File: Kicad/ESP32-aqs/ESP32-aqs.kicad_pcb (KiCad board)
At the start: 2 copper layers, 22 parts, among them J1 UART Connector, J2 Conn SEN55, J3 ufl connector, U1 LD1117S33TR_SOT223, U2 ESP32-WROOM-32, U3 SGP41-D-R4, U4 SX1276S8S+T-X1

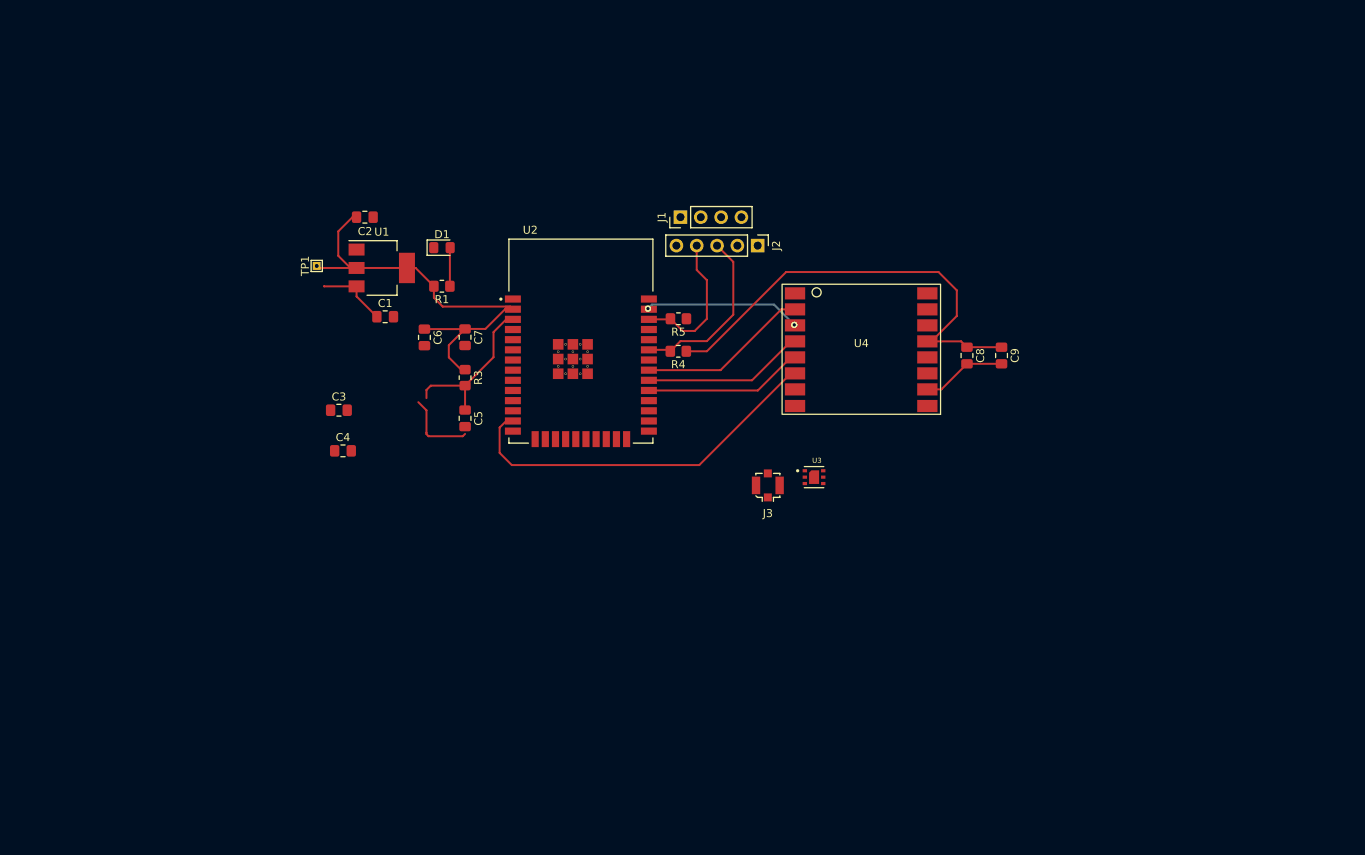
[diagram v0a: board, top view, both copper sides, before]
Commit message: PCB design update
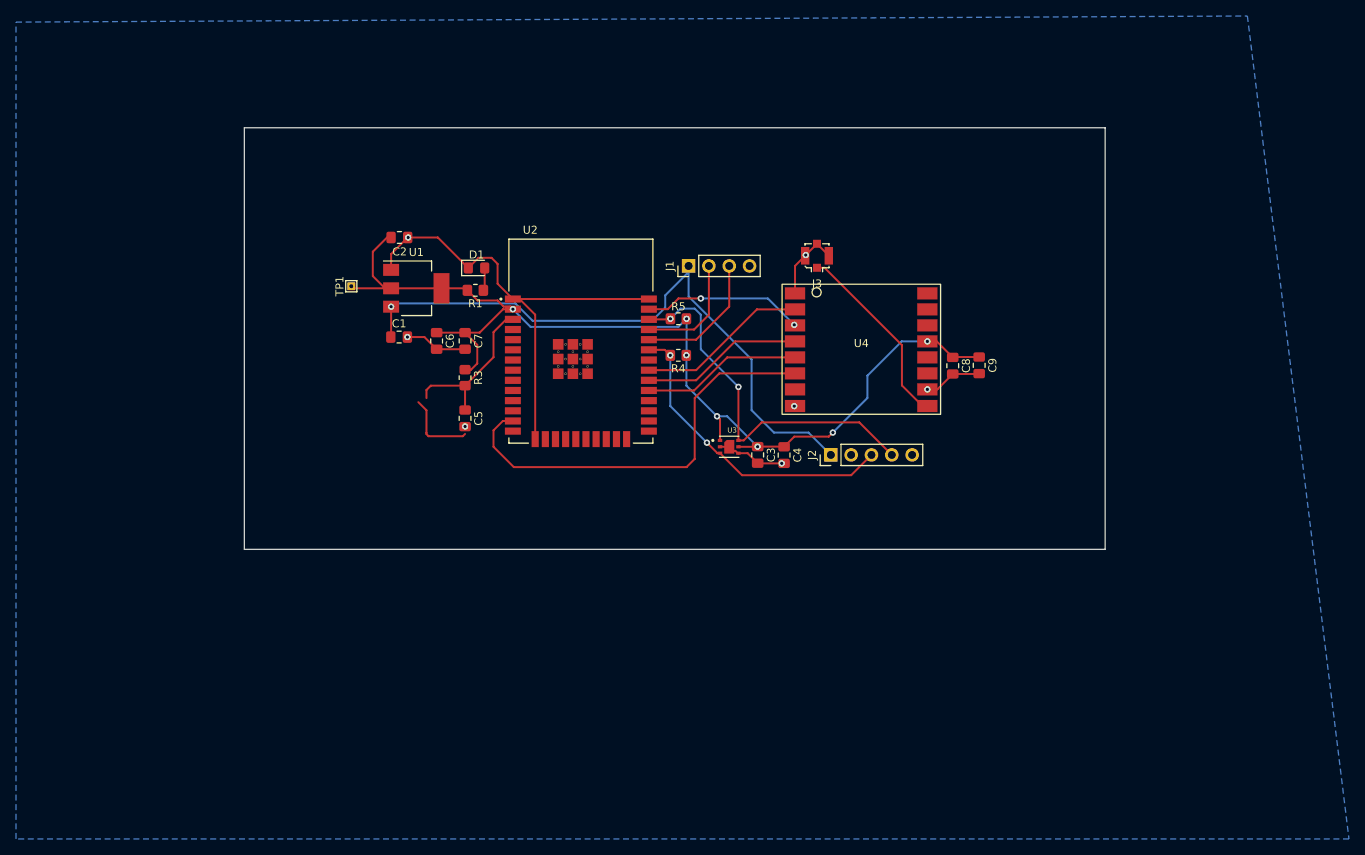
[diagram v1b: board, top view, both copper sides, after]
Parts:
- moved C4 55.1 mm to (182.4, 101.6), turned to -90 degrees
- moved C3 52.6 mm to (179.1, 101.6), turned to -90 degrees
- moved J3 29.4 mm to (186.5, 76.7)
- moved J2 27.7 mm to (188.2, 101.6), turned to 90 degrees
- moved U3 11.3 mm to (175.5, 100.6)
- moved J1 6.18 mm to (170.4, 78.0)
- moved D1 5.01 mm to (143.9, 78.2)
- moved TP1 5.01 mm to (128.3, 80.5)
- moved C2 5.01 mm to (134.3, 74.4)
- moved U1 5.01 mm to (136.4, 80.8)
- moved R1 4.21 mm to (143.8, 81.0)
- moved C1 3.08 mm to (134.2, 86.9)
- moved C9 3.05 mm to (206.8, 90.4)
- moved C8 2.18 mm to (203.5, 90.4)
- moved C6 1.59 mm to (138.9, 87.4)
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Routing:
- net GND: track 10.6 -> 92.6 mm, vias 0 -> 7
- net VIN: track 8.92 -> 79.8 mm, vias 0 -> 1
- net SCL: track 18.2 -> 46.8 mm, vias 0 -> 2
- net Net-(J3-Pad1): track 0.00 -> 23.9 mm
- net +3V3: track 112.4 -> 132.2 mm, vias 0 -> 7
- net SDA: track 22.0 -> 39.1 mm, vias 0 -> 2
- net TX: track 0.00 -> 16.8 mm
- net RX: track 0.00 -> 14.4 mm
- net RST: track 47.5 -> 53.0 mm
- net Net-(D1-Pad2): track 4.84 -> 2.86 mm
- net MOSI: track 19.6 -> 20.1 mm
- added copper zone on B.Cu, net GND
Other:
- board outline added: 107.6 x 52.7 mm

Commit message: PCB design
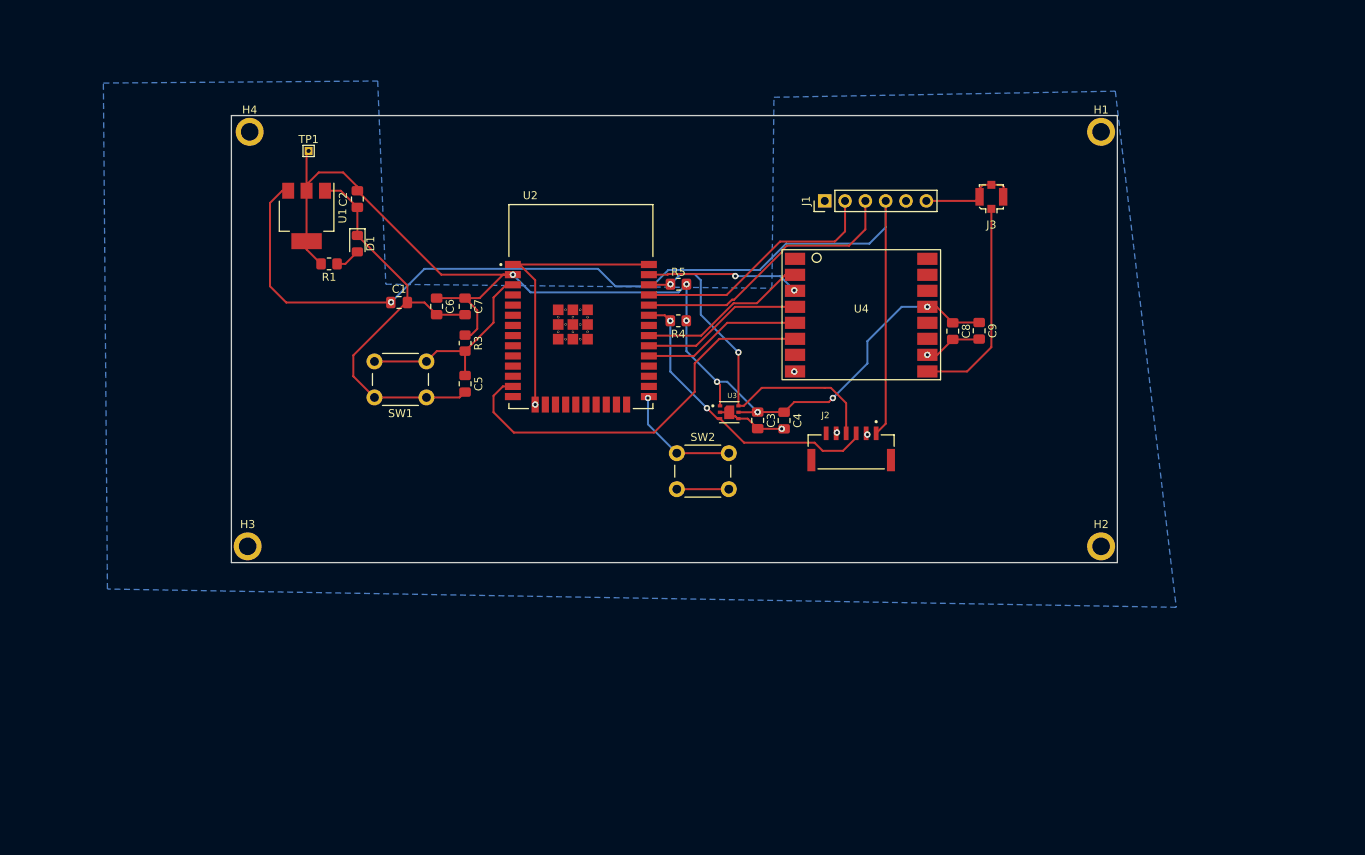
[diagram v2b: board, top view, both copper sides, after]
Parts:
- added H1: MountingHole, MountingHole:MountingHole_2.2mm_M2_ISO7380_Pad, F.Cu at (222.0, 61.2)
- added H2: MountingHole, MountingHole:MountingHole_2.2mm_M2_ISO7380_Pad, F.Cu at (222.0, 113.0)
- added H3: MountingHole, MountingHole:MountingHole_2.2mm_M2_ISO7380_Pad, F.Cu at (115.3, 113.0)
- added H4: MountingHole, MountingHole:MountingHole_2.2mm_M2_ISO7380_Pad, F.Cu at (115.6, 61.2)
- added SW1: RESET, Button_Switch_THT:SW_PUSH_6mm_H7.3mm, F.Cu at (137.7, 94.4)
- added SW2: BOOT, Button_Switch_THT:SW_PUSH_6mm_H7.3mm, F.Cu at (169.0, 101.4)
- J1: footprint Connector_PinHeader_2.54mm:PinHeader_1x04_P2.54mm_Vertical -> Connector_PinHeader_2.54mm:PinHeader_1x06_P2.54mm_Vertical
- J2: value Conn SEN55 -> JST connector SEN55; footprint Connector_PinHeader_2.54mm:PinHeader_1x05_P2.54mm_Vertical -> ESP32-aqs:JST_BM06B-GHS-TBT_LF__SN__N_
- moved J3 23.0 mm to (208.3, 69.3)
- moved J1 18.9 mm to (187.5, 69.8)
- moved R1 18.6 mm to (125.5, 77.7)
- moved TP1 17.7 mm to (122.9, 63.6), turned to 0 degrees
- moved U1 16.4 mm to (122.7, 71.7), turned to -90 degrees
- moved D1 15.2 mm to (129.0, 75.2), turned to -90 degrees
- moved C2 7.12 mm to (129.0, 69.6), turned to -90 degrees
- moved C5 4.32 mm to (142.5, 92.7)
- moved C1 4.32 mm to (134.2, 82.5)
- moved C3 4.32 mm to (179.1, 97.3)
- moved C4 4.32 mm to (182.4, 97.3)
- moved C6 4.32 mm to (138.9, 83.0)
- moved C7 4.32 mm to (142.5, 83.0)
- moved C8 4.32 mm to (203.5, 86.1)
- moved C9 4.32 mm to (206.8, 86.1)
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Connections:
- J1 pad 1: VIN -> unconnected-(J1-Pad1)
- J1 pad 4: GND -> VIN
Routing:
- net VIN: track 79.8 -> 129.7 mm
- net GND: track 92.6 -> 125.3 mm, vias 7 -> 6
- net TX: track 16.8 -> 34.6 mm
- net +3V3: track 132.2 -> 149.5 mm
- net RX: track 14.4 -> 31.6 mm
- net BOOT: track 0.00 -> 14.9 mm, vias 0 -> 1
- net (no net): track 9.47 -> 0.00 mm
- net EN: track 20.4 -> 26.2 mm
- net SCL: track 46.8 -> 44.0 mm
- net Net-(J3-Pad1): track 23.9 -> 26.6 mm
- net RST: track 53.0 -> 50.6 mm
- net SDA: track 39.1 -> 37.9 mm
- net MOSI: track 20.1 -> 19.0 mm
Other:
- board size 107.6 x 52.7 mm -> 110.7 x 55.9 mm
